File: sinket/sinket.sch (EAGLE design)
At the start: 21 parts, among them IC1 ATTINY85-20PU, IC2 TS2940CP50S

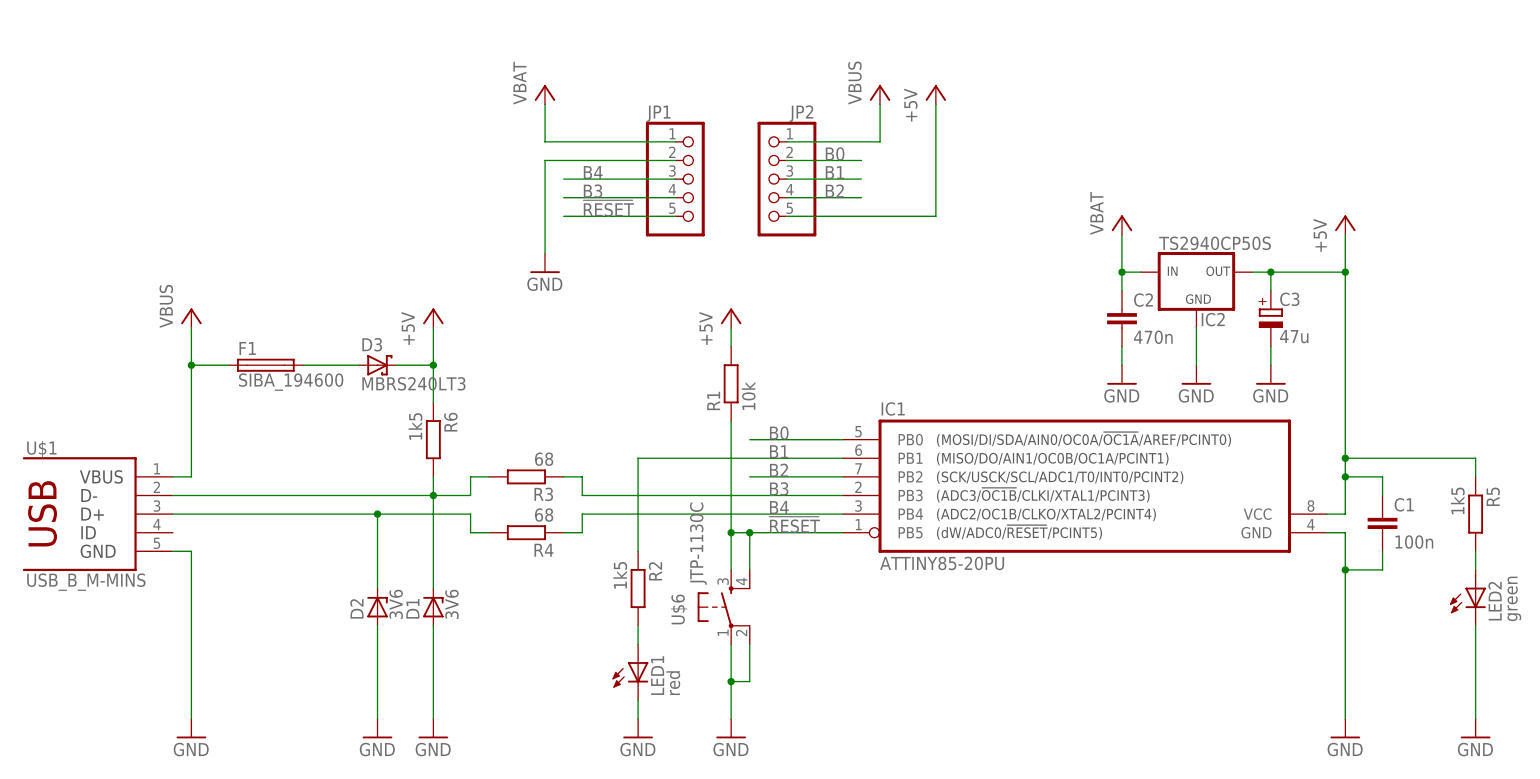
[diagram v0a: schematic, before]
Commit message: change fuse package
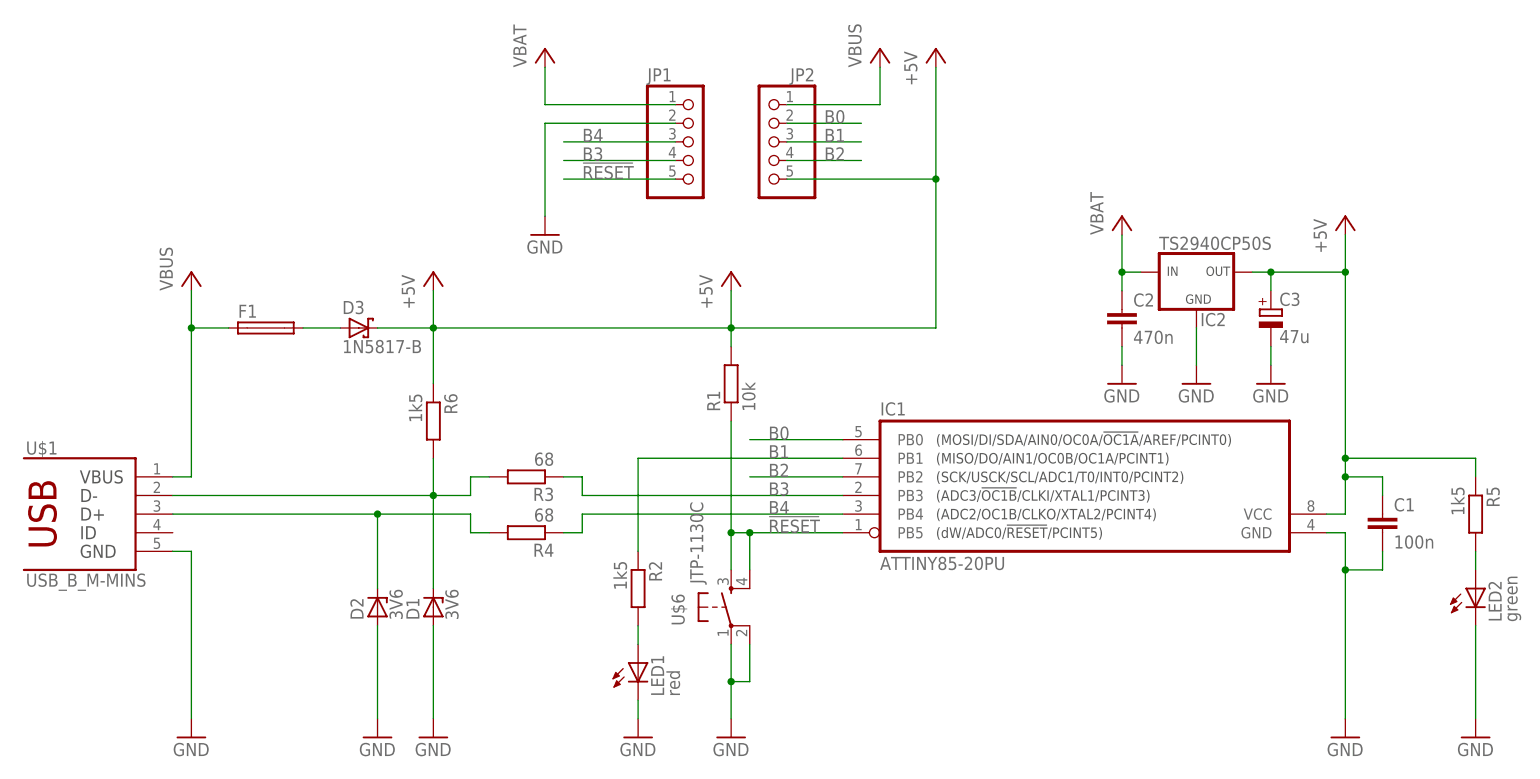
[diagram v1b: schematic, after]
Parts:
- D3: value MBRS240LT3 -> 1N5817-B; device diode:MBRS130LT3 -> diode:1N5817-B
- F1: value SIBA_194600 -> (none); device n39:SIBA_194600 -> n39:PTC-FUSE-LP60-050
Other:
- moved on the sheet: D3, F1, JP1, JP2, R6
